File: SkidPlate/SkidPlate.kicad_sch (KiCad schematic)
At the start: 38 parts, among them J1 conn, J2 conn, J3 conn, J4 conn, J5 conn, J6 conn, J7 conn, J8 S4B-PH-SM4-TB, U2 LSM6DSOX, U3 IC_PMW3360DM-T2QU

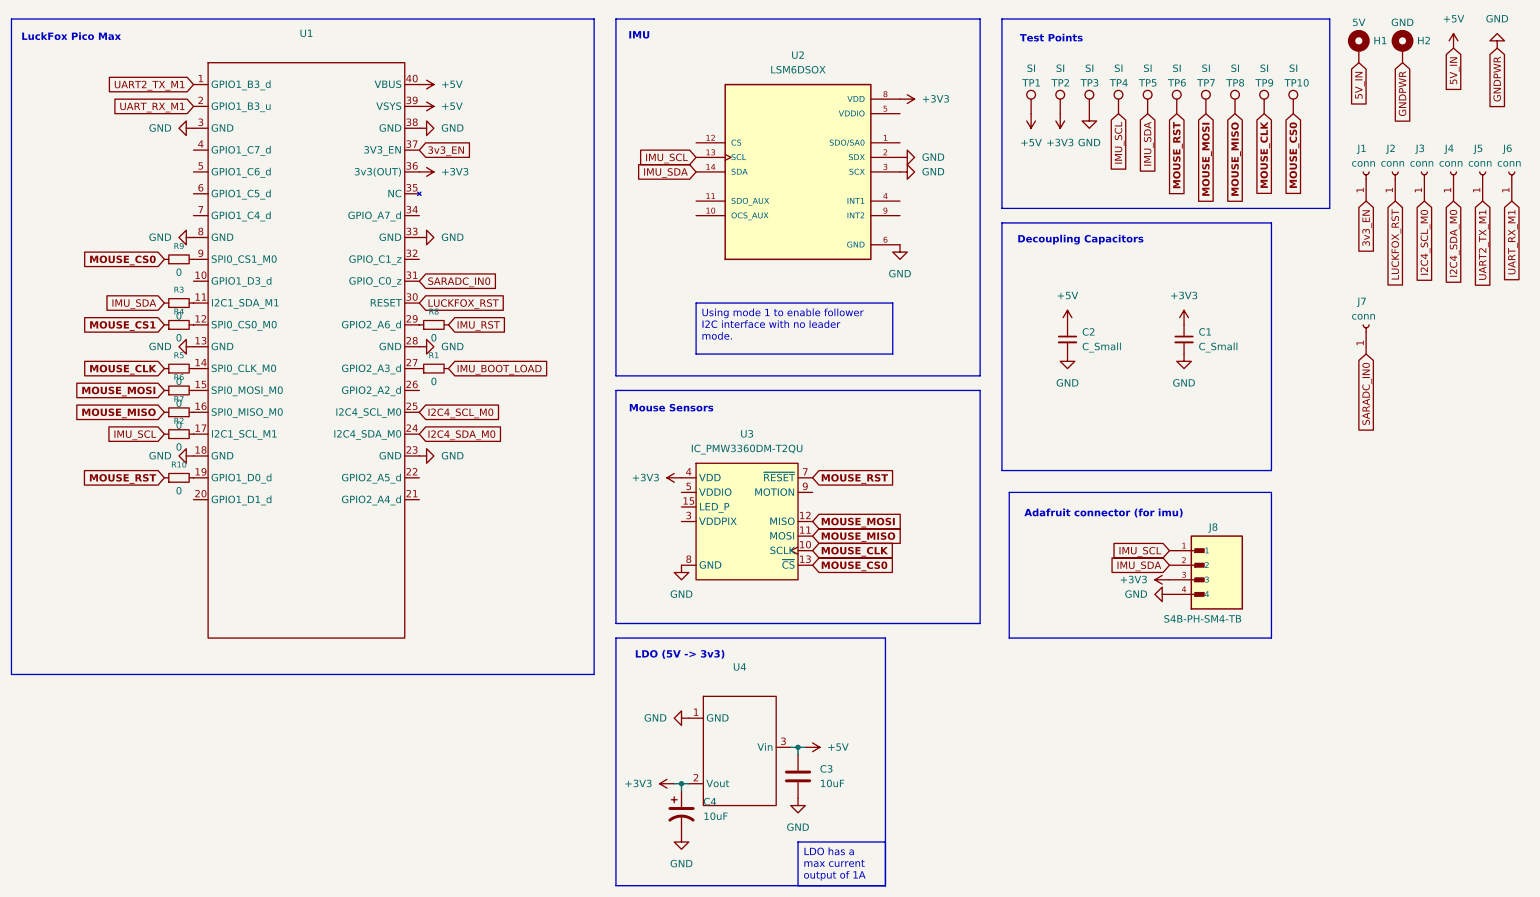
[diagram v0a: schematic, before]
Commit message: midplate additions WIP
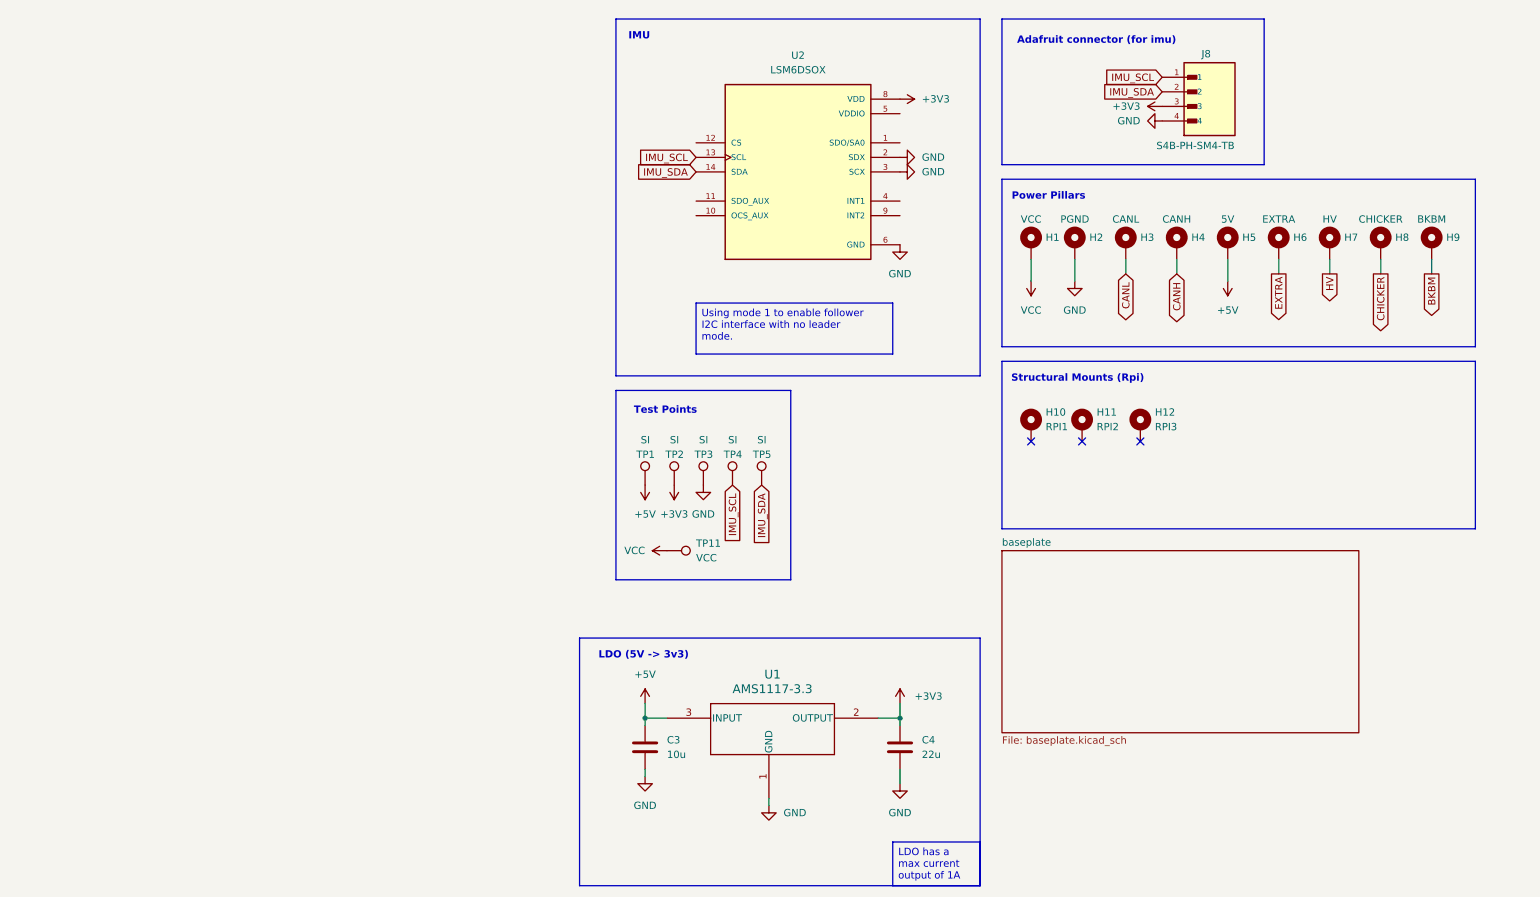
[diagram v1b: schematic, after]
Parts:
- removed C1, C2: C_Small, bots:C_0603_1608Metric, symbol Device:C_Small
- removed C3: 10uF, Capacitor_SMD:C_1206_3216Metric, symbol Device:C
- removed C4: 10uF, bots:CAP_25SVPF100M, symbol bots:C_1000u_POL
- removed J1, J2, J3, J4, J5, J6, J7: conn, symbol Connector:Conn_01x01_Socket
- removed R1, R10, R2, R3, R4, R5, R6, R7, R8, R9: 0, bots:R_0603_1608Metric, symbol Device:R_Small
- removed TP10, TP6, TP7, TP8, TP9: SI, bots:pad_0603, symbol bots:TestPoint_1x1
- removed U1: ~, bots:RV1106_PICO_MAX, symbol bots:RV1106_PICO_MAX
- removed U3: IC_PMW3360DM-T2QU, bots:IC_PMW3360DM-T2QU 16Pin, symbol bots:IC_PMW3360DM-T2QU
- removed U4: ~, Package_TO_SOT_SMD:SOT-223, symbol bots:BL1117-33-A-SOT-223
- added C3: 10u, bots:C_0805_2012Metric, symbol bots:C_10u
- added C4: 22u, bots:C_0603_1608Metric, symbol bots:C_22u
- added H10: RPI1, bots:MountingHole_2.7mm_M2.5_DIN965_Pad, symbol bots:MountingHoleM2.5NoThread_wConn
- added H11: RPI2, bots:MountingHole_2.7mm_M2.5_DIN965_Pad, symbol bots:MountingHoleM2.5NoThread_wConn
- added H12: RPI3, bots:MountingHole_2.7mm_M2.5_DIN965_Pad, symbol bots:MountingHoleM2.5NoThread_wConn
- added H3: CANL, bots:MountingHole_2.7mm_M2.5_DIN965_Pad, symbol bots:MountingHoleM2.5NoThread_wConn
- added H4: CANH, bots:MountingHole_2.7mm_M2.5_DIN965_Pad, symbol bots:MountingHoleM2.5NoThread_wConn
- added H5: 5V, bots:MountingHole_2.7mm_M2.5_DIN965_Pad, symbol bots:MountingHoleM2.5NoThread_wConn
- added H6: EXTRA, bots:MountingHole_2.7mm_M2.5_DIN965_Pad, symbol bots:MountingHoleM2.5NoThread_wConn
- added H7: HV, bots:MountingHole_2.7mm_M2.5_DIN965_Pad, symbol bots:MountingHoleM2.5NoThread_wConn
- added H8: CHICKER, bots:MountingHole_2.7mm_M2.5_DIN965_Pad, symbol bots:MountingHoleM2.5NoThread_wConn
- added H9: BKBM, bots:MountingHole_2.7mm_M2.5_DIN965_Pad, symbol bots:MountingHoleM2.5NoThread_wConn
- added TP11: VCC, bots:TestPoint_Pad_2.0x2.0mm, symbol bots:TestPoint_2x2
- added U1: AMS1117-3.3, bots:SOT-223-3_TabPin2, symbol bots:AMS1117-3.3
- H1: value 5V -> VCC
- H2: value GND -> PGND
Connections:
- net +3V3: now also C4.1, U1.2 (OUTPUT)
- net +5V: now also C3.1, H5.1, U1.3 (INPUT); no longer H1.1
- net GND: now also C3.2, C4.2, U1.1 (GND)
- new net BKBM: H9.1
- new net CANH: H4.1
- new net CANL: H3.1
- new net CHICKER: H8.1
- new net EXTRA: H6.1
- new net HV: H7.1
- new net VCC: H1.1, TP11.1
- no-connect marks 0 -> 3
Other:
- added sheet baseplate (baseplate.kicad_sch)
- note added: "Power Pillars"
- note added: "Structural Mounts (Rpi)"
- note removed: "Decoupling Capacitors"
- note removed: "LuckFox Pico Max"
- note removed: "Mouse Sensors"
- moved on the sheet: J8, TP1, TP2, TP3, TP4, TP5
